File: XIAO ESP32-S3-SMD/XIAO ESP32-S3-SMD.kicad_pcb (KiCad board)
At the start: 2 copper layers, 34.6 x 37.9 mm, 12 parts, among them U2 XIAO-ESP32-S3-SMD

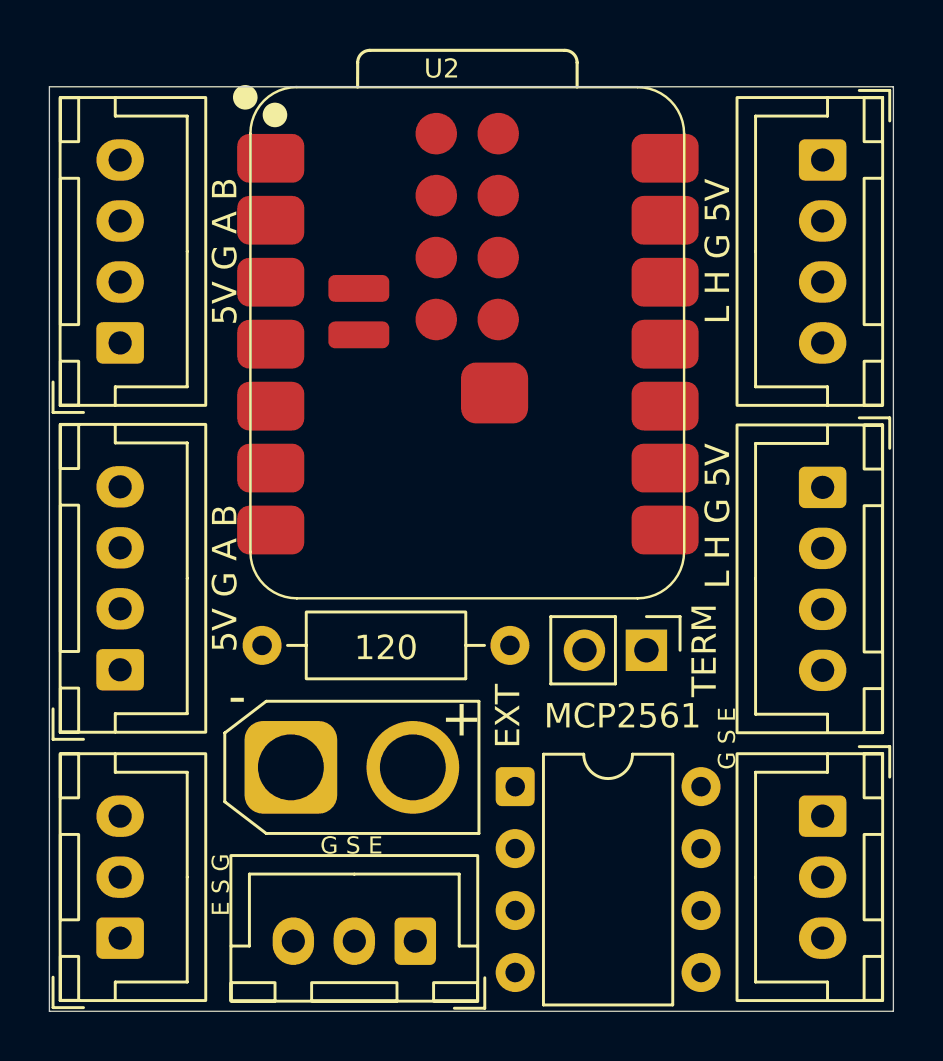
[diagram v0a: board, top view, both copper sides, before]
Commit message: 電源ラインの配線
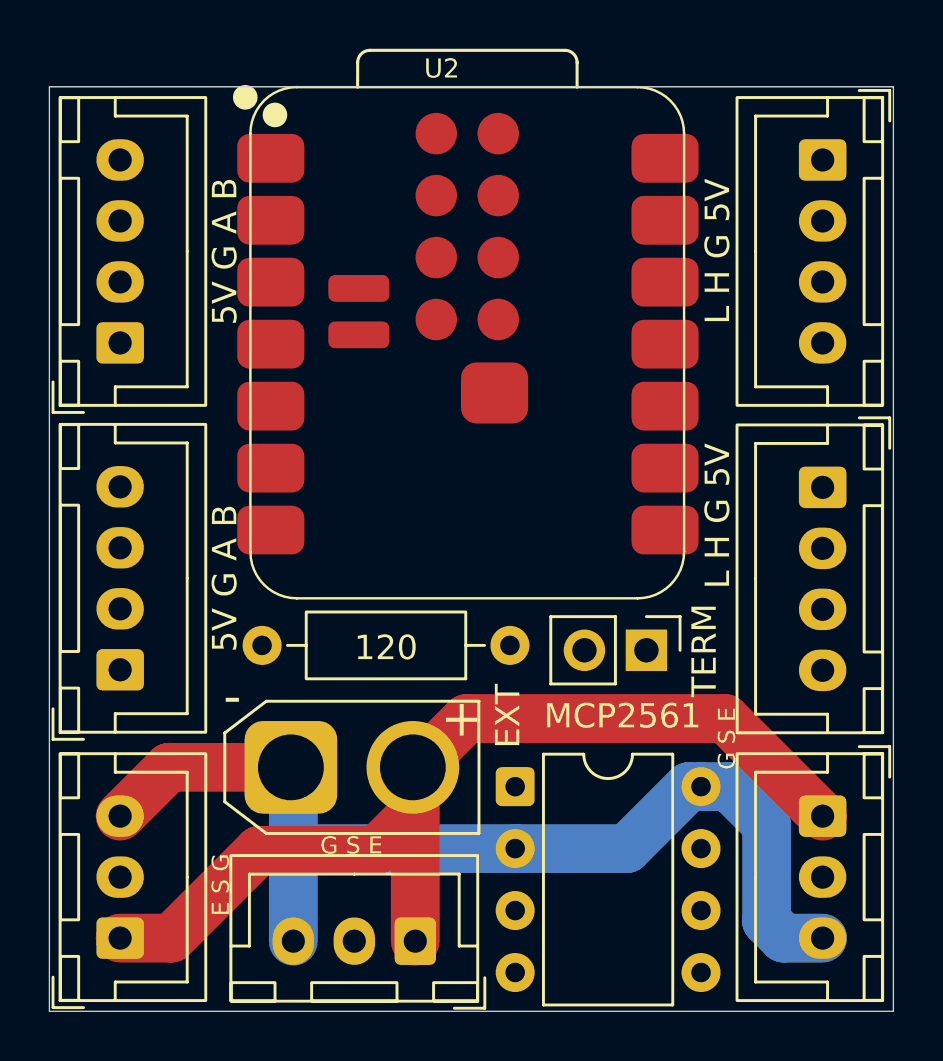
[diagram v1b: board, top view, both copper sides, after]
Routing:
- net GND: track 0.00 -> 42.6 mm
- net EXT_POWER: track 0.00 -> 42.4 mm
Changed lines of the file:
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@@
 		)
 		(fp_text user "-"
-			(at -2.2 -2.9 0)
+			(at -2.4 -2.9 0)
 			(layer "F.SilkS")
 			(effects
@@
 		)
 	)
+	(segment
+		(start 137.6 90.3)
+		(end 135.6 92.3)
+		(width 2)
+		(layer "F.Cu")
+		(net "GND")
+	)
+	(segment
+		(start 142.6 90.3)
+		(end 137.6 90.3)
+		(width 2)
+		(layer "F.Cu")
+		(net "GND")
+	)
+	(segment
+		(start 142.73 93.63)
+		(end 142.7 93.6)
+		(width 2)
+		(layer "B.Cu")
+		(net "GND")
+	)
+	(segment
+		(start 151.795 93.63)
+		(end 142.73 93.63)
+		(width 2)
+		(layer "B.Cu")
+		(net "GND")
+	)
+	(segment
+		(start 164.4 97.3)
+		(end 162.8 97.3)
+		(width 2)
+		(layer "B.Cu")
+		(net "GND")
+	)
+	(segment
+		(start 142.7 93.6)
+		(end 142.7 90.4)
+		(width 2)
+		(layer "B.Cu")
+		(net "GND")
+	)
+	(segment
+		(start 158.91 91.09)
+		(end 156.37 93.63)
+		(width 2)
+		(layer "B.Cu")
+		(net "GND")
+	)
+	(segment
+		(start 142.7 97.425)
+		(end 142.7 93.6)
+		(width 2)
+		(layer "B.Cu")
+		(net "GND")
+	)
+	(segment
+		(start 142.7 90.4)
+		(end 142.6 90.3)
+		(width 0.2)
+		(layer "B.Cu")
+		(net "GND")
+	)
+	(segment
+		(start 160.54637 91.09)
+		(end 159.415 91.09)
+		(width 2)
+		(layer "B.Cu")
+		(net "GND")
+	)
+	(segment
+		(start 159.415 91.09)
+		(end 158.91 91.09)
+		(width 2)
+		(layer "B.Cu")
+		(net "GND")
+	)
+	(segment
+		(start 162.8 97.3)
+		(end 162.1 96.6)
+		(width 2)
+		(layer "B.Cu")
+		(net "GND")
+	)
+	(segment
+		(start 156.37 93.63)
+		(end 151.795 93.63)
+		(width 2)
+		(layer "B.Cu")
+		(net "GND")
+	)
+	(segment
+		(start 162.1 96.6)
+		(end 162.1 92.64363)
+		(width 2)
+		(layer "B.Cu")
+		(net "GND")
+	)
+	(segment
+		(start 162.1 92.64363)
+		(end 160.54637 91.09)
+		(width 2)
+		(layer "B.Cu")
+		(net "GND")
+	)
+	(segment
+		(start 135.6 97.3)
+		(end 137.7 97.3)
+		(width 2)
+		(layer "F.Cu")
+		(net "EXT_POWER")
+	)
+	(segment
+		(start 147.7 97.425)
+		(end 147.7 90.4)
+		(width 2)
+		(layer "F.Cu")
+		(net "EXT_POWER")
+	)
+	(segment
+		(start 147.7 90.4)
+		(end 147.6 90.3)
+		(width 0.2)
+		(layer "F.Cu")
+		(net "EXT_POWER")
+	)
+	(segment
+		(start 141.3 93.7)
+		(end 146.1 93.7)
+		(width 2)
+		(layer "F.Cu")
+		(net "EXT_POWER")
+	)
+	(segment
+		(start 147.7 90.4)
+		(end 149.8 88.3)
+		(width 2)
+		(layer "F.Cu")
+		(net "EXT_POWER")
+	)
+	(segment
+		(start 137.7 97.3)
+		(end 141.3 93.7)
+		(width 2)
+		(layer "F.Cu")
+		(net "EXT_POWER")
+	)
+	(segment
+		(start 146.1 93.7)
+		(end 147.6 92.2)
+		(width 2)
+		(layer "F.Cu")
+		(net "EXT_POWER")
+	)
+	(segment
+		(start 147.6 92.2)
+		(end 147.6 90.3)
+		(width 0.2)
+		(layer "F.Cu")
+		(net "EXT_POWER")
+	)
+	(segment
+		(start 160.4 88.3)
+		(end 164.4 92.3)
+		(width 2)
+		(layer "F.Cu")
+		(net "EXT_POWER")
+	)
+	(segment
+		(start 149.8 88.3)
+		(end 160.4 88.3)
+		(width 2)
+		(layer "F.Cu")
+		(net "EXT_POWER")
+	)
 	(embedded_fonts no)
